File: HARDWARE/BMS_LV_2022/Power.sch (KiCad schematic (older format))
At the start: 19 parts, among them U2 LM1117-3.3, U3 LMR23610

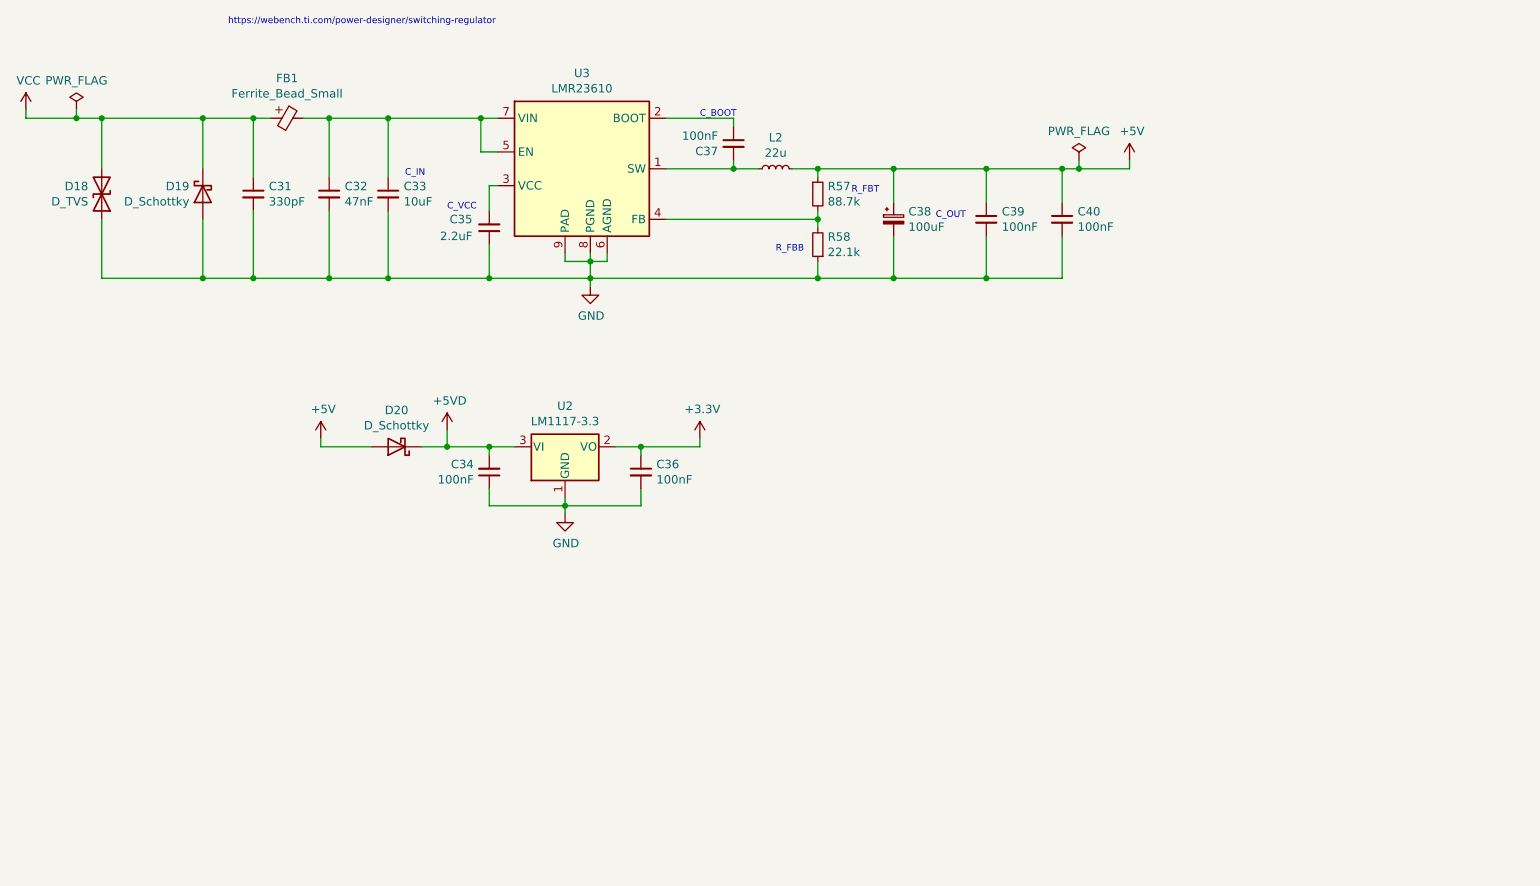
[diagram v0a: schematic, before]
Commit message: Most of the footprints added
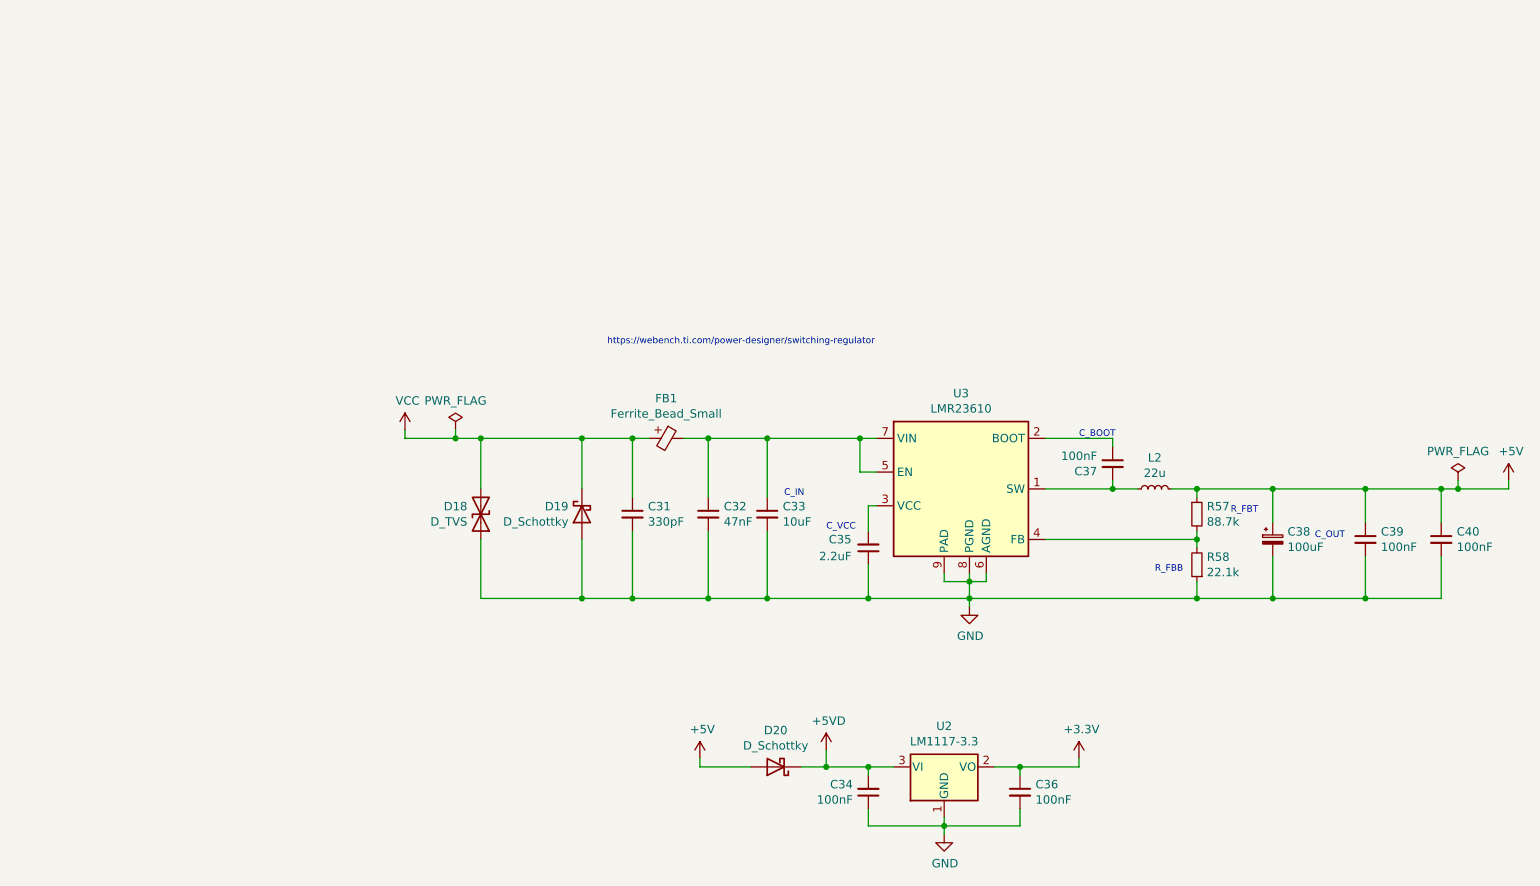
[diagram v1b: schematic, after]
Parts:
- C31, C32, C33, C34, C35, C36, C37, C39, C40: footprint (none) -> Capacitor_SMD:C_0603_1608Metric
- C38: footprint (none) -> Capacitor_SMD:CP_Elec_6.3x7.7
- D18, D19, D20: footprint (none) -> Diode_SMD:D_SMB
- FB1: footprint (none) -> Inductor_SMD:L_0603_1608Metric
- L2: footprint (none) -> Inductor_SMD:L_12x12mm_H8mm
- R57, R58: footprint (none) -> Resistor_SMD:R_0603_1608Metric
- U2: footprint (none) -> Package_TO_SOT_SMD:SOT-223-3_TabPin2
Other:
- moved on the sheet: C31, C32, C33, C34, C35, C36, C37, C38, C39, C40, D18, D19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

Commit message: Some footprint changes
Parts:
- D20: footprint Diode_SMD:D_SMB -> Diode_SMD:D_SOD-123
- FB1: symbol FerriteBead:Ferrite_Bead_Small -> BMS_LV_2022-rescue:Ferrite_Bead_Small-FerriteBead
- L2: footprint Inductor_SMD:L_12x12mm_H8mm -> Inductor_SMD:L_6.3x6.3_H3
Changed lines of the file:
@@
 F 0 "L2" V 7585 3650 50  0000 C CNN
 F 1 "22u" V 7494 3650 50  0000 C CNN
-F 2 "Inductor_SMD:L_12x12mm_H8mm" H 7400 3650 50  0001 C CNN
+F 2 "Inductor_SMD:L_6.3x6.3_H3" H 7400 3650 50  0001 C CNN
 F 3 "~" H 7400 3650 50  0001 C CNN
 	1    7400 3650
@@
 Connection ~ 8650 3650
 $Comp
-L FerriteBead:Ferrite_Bead_Small FB1
+L BMS_LV_2022-rescue:Ferrite_Bead_Small-FerriteBead FB1
 U 1 1 61BEAA28
 P 4500 3350
+AR Path="/61BEAA28" Ref="FB1"  Part="1"
+AR Path="/61D97AE8/61BEAA28" Ref="FB1"  Part="1"
 F 0 "FB1" V 4263 3350 50  0000 C CNN
 F 1 "Ferrite_Bead_Small" V 4354 3350 50  0000 C CNN
@@
 F 0 "D20" H 5150 5083 50  0000 C CNN
 F 1 "D_Schottky" H 5150 5174 50  0000 C CNN
-F 2 "Diode_SMD:D_SMB" H 5150 5300 50  0001 C CNN
+F 2 "Diode_SMD:D_SOD-123" H 5150 5300 50  0001 C CNN
 F 3 "~" H 5150 5300 50  0001 C CNN
 	1    5150 5300
